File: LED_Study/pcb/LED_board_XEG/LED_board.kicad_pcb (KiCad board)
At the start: 2 copper layers, 25.4 x 25.4 mm, 4 parts

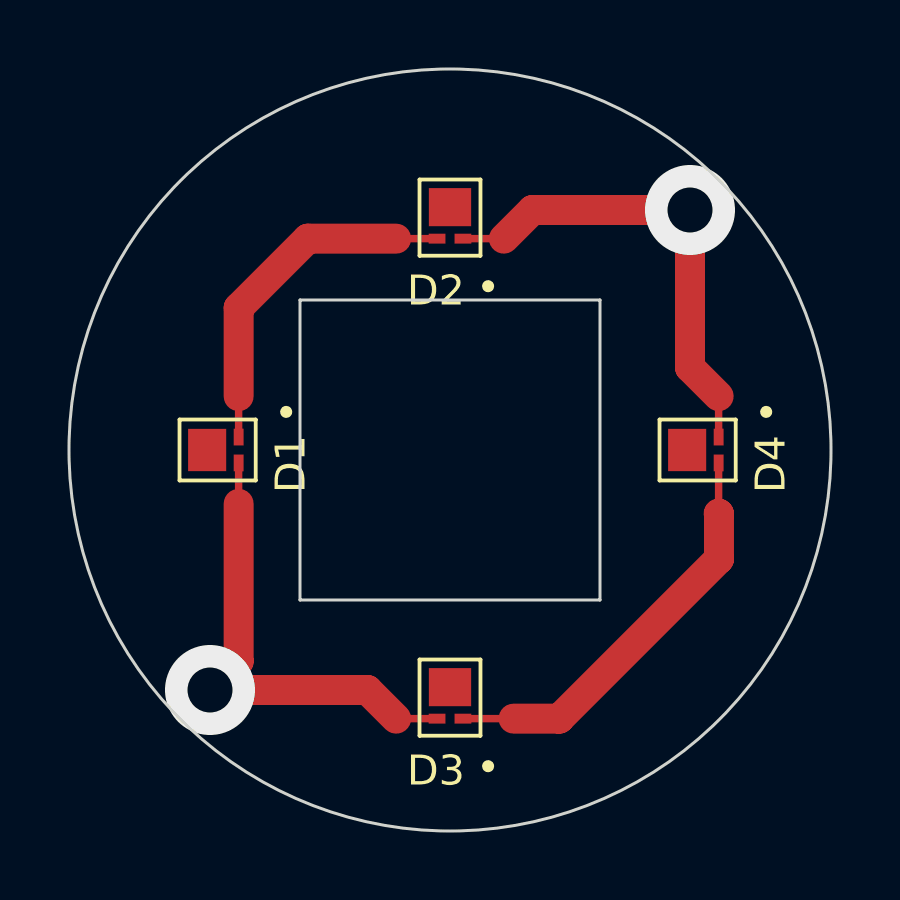
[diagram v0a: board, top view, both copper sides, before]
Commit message: new boards
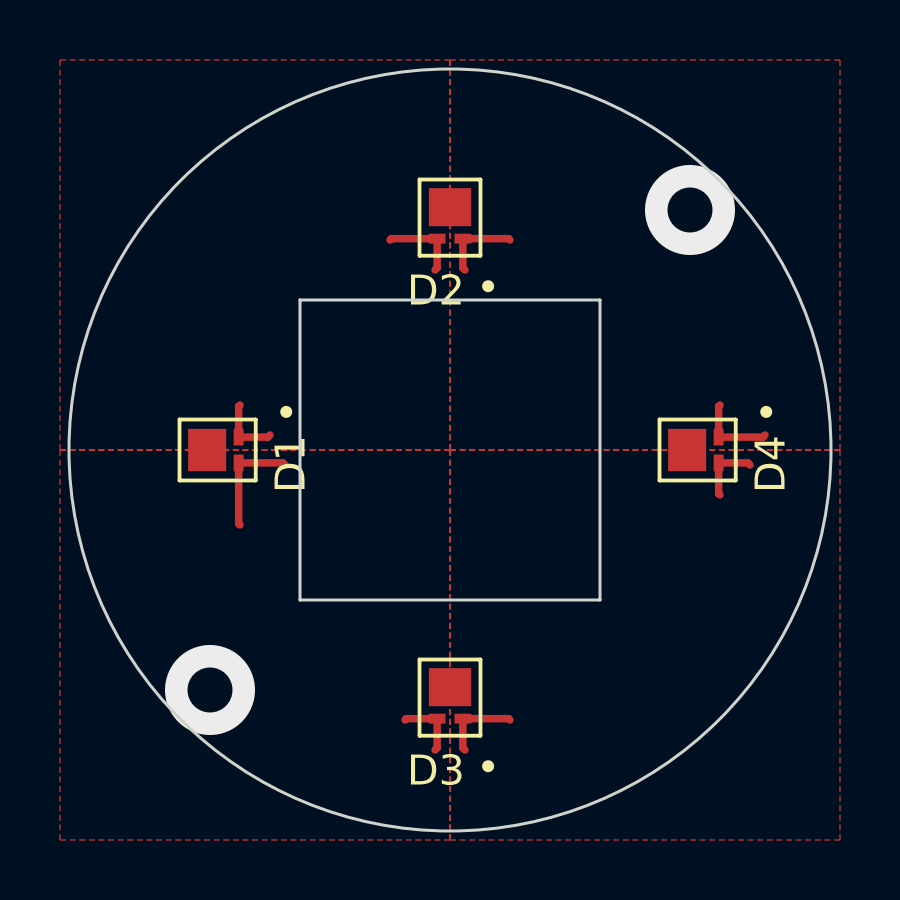
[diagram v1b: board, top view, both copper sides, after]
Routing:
- net /GND: track 15.9 -> 5.33 mm
- net /Vin: track 15.9 -> 5.83 mm
- net Net-(D3-Pad1): track 13.9 -> 4.83 mm
- net Net-(D1-Pad1): track 11.9 -> 4.83 mm
- added copper zone on F.Cu, net /GND
- added copper zone on F.Cu, net /Vin
- added copper zone on F.Cu, net Net-(D1-Pad1)
- added copper zone on F.Cu, net Net-(D3-Pad1)
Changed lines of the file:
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@@
   (gr_circle (center 100 100) (end 112.7 100)
     (stroke (width 0.1) (type default)) (fill none) (layer "Edge.Cuts"))
-  (segment (start 92.955 95.259) (end 95.259 92.955) (width 1) (layer "F.Cu") (net 1))
-  (segment (start 95.259 92.955) (end 98.205 92.955) (width 1) (layer "F.Cu") (net 1))
-  (segment (start 99.57 92.955) (end 98.205 92.955) (width 0.25) (layer "F.Cu") (net 1))
-  (segment (start 92.955 99.57) (end 92.955 98.205) (width 0.25) (layer "F.Cu") (net 1))
-  (segment (start 92.955 98.205) (end 92.955 95.259) (width 1) (layer "F.Cu") (net 1))
-  (segment (start 98.205 108.955) (end 97.25 108) (width 1) (layer "F.Cu") (net 3))
-  (segment (start 92.955 101.795) (end 92.955 107.045) (width 1) (layer "F.Cu") (net 3))
-  (segment (start 92.955 107.045) (end 92 108) (width 1) (layer "F.Cu") (net 3))
-  (segment (start 92.955 100.43) (end 92.955 101.795) (width 0.25) (layer "F.Cu") (net 3))
-  (segment (start 97.25 108) (end 92 108) (width 1) (layer "F.Cu") (net 3))
-  (segment (start 99.57 108.955) (end 98.205 108.955) (width 0.25) (layer "F.Cu") (net 3))
+  (segment (start 99.57 92.955) (end 99.57 93.93) (width 0.25) (layer "F.Cu") (net 1))
+  (segment (start 92.955 98.545) (end 93 98.5) (width 0.25) (layer "F.Cu") (net 1))
+  (segment (start 92.955 99.57) (end 92.955 98.545) (width 0.25) (layer "F.Cu") (net 1))
+  (segment (start 99.57 93.93) (end 99.5 94) (width 0.25) (layer "F.Cu") (net 1))
+  (segment (start 98.045 92.955) (end 98 93) (width 0.25) (layer "F.Cu") (net 1))
+  (segment (start 93.93 99.57) (end 94 99.5) (width 0.25) (layer "F.Cu") (net 1))
+  (segment (start 92.955 99.57) (end 93.93 99.57) (width 0.25) (layer "F.Cu") (net 1))
+  (segment (start 99.57 92.955) (end 98.045 92.955) (width 0.25) (layer "F.Cu") (net 1))
+  (segment (start 99.57 108.955) (end 98.545 108.955) (width 0.25) (layer "F.Cu") (net 3))
+  (segment (start 94.43 100.43) (end 94.5 100.5) (width 0.25) (layer "F.Cu") (net 3))
+  (segment (start 98.545 108.955) (end 98.5 109) (width 0.25) (layer "F.Cu") (net 3))
+  (segment (start 92.955 100.43) (end 94.43 100.43) (width 0.25) (layer "F.Cu") (net 3))
+  (segment (start 92.955 100.43) (end 92.955 102.455) (width 0.25) (layer "F.Cu") (net 3))
+  (segment (start 99.57 108.955) (end 99.57 109.93) (width 0.25) (layer "F.Cu") (net 3))
+  (segment (start 99.57 109.93) (end 99.5 110) (width 0.25) (layer "F.Cu") (net 3))
+  (segment (start 92.955 102.455) (end 93 102.5) (width 0.25) (layer "F.Cu") (net 3))
   (via (at 92 108) (size 3) (drill 1.5) (layers "F.Cu" "B.Cu") (free) (net 3))
-  (segment (start 108 92) (end 102.75 92) (width 1) (layer "F.Cu") (net 4))
-  (segment (start 108 92) (end 108 97.25) (width 1) (layer "F.Cu") (net 4))
-  (segment (start 108.955 98.205) (end 108 97.25) (width 1) (layer "F.Cu") (net 4))
-  (segment (start 101.795 92.955) (end 102.75 92) (width 1) (layer "F.Cu") (net 4))
-  (segment (start 108.955 99.57) (end 108.955 98.205) (width 0.25) (layer "F.Cu") (net 4))
-  (segment (start 100.43 92.955) (end 101.795 92.955) (width 0.25) (layer "F.Cu") (net 4))
+  (segment (start 100.43 92.955) (end 100.43 93.93) (width 0.25) (layer "F.Cu") (net 4))
+  (segment (start 108.955 99.57) (end 110.43 99.57) (width 0.25) (layer "F.Cu") (net 4))
+  (segment (start 108.955 98.545) (end 109 98.5) (width 0.25) (layer "F.Cu") (net 4))
+  (segment (start 100.43 93.93) (end 100.5 94) (width 0.25) (layer "F.Cu") (net 4))
+  (segment (start 100.43 92.955) (end 101.955 92.955) (width 0.25) (layer "F.Cu") (net 4))
+  (segment (start 110.43 99.57) (end 110.5 99.5) (width 0.25) (layer "F.Cu") (net 4))
+  (segment (start 101.955 92.955) (end 102 93) (width 0.25) (layer "F.Cu") (net 4))
+  (segment (start 108.955 99.57) (end 108.955 98.545) (width 0.25) (layer "F.Cu") (net 4))
   (via (at 108 92) (size 3) (drill 1.5) (layers "F.Cu" "B.Cu") (free) (net 4))
-  (segment (start 108.966 103.632) (end 103.643 108.955) (width 1) (layer "F.Cu") (net 6))
-  (segment (start 108.966 102.13) (end 108.966 103.632) (width 1) (layer "F.Cu") (net 6))
-  (segment (start 100.43 108.955) (end 102.119 108.955) (width 0.25) (layer "F.Cu") (net 6))
-  (segment (start 108.955 102.119) (end 108.966 102.13) (width 1) (layer "F.Cu") (net 6))
-  (segment (start 108.955 100.43) (end 108.955 102.119) (width 0.25) (layer "F.Cu") (net 6))
-  (segment (start 103.643 108.955) (end 102.119 108.955) (width 1) (layer "F.Cu") (net 6))
+  (segment (start 100.43 108.955) (end 100.43 109.93) (width 0.25) (layer "F.Cu") (net 6))
+  (segment (start 108.955 101.455) (end 109 101.5) (width 0.25) (layer "F.Cu") (net 6))
+  (segment (start 101.955 108.955) (end 102 109) (width 0.25) (layer "F.Cu") (net 6))
+  (segment (start 109.93 100.43) (end 110 100.5) (width 0.25) (layer "F.Cu") (net 6))
+  (segment (start 100.43 108.955) (end 101.955 108.955) (width 0.25) (layer "F.Cu") (net 6))
+  (segment (start 108.955 100.43) (end 109.93 100.43) (width 0.25) (layer "F.Cu") (net 6))
+  (segment (start 108.955 100.43) (end 108.955 101.455) (width 0.25) (layer "F.Cu") (net 6))
+  (segment (start 100.43 109.93) (end 100.5 110) (width 0.25) (layer "F.Cu") (net 6))
+  (zone (net 1) (net_name "Net-(D1-Pad1)") (layer "F.Cu") (hatch edge 0.5)
+    (priority 3)
+    (connect_pads (clearance 0.5))
+    (min_thickness 0.25) (filled_areas_thickness no)
+    (fill yes (thermal_gap 0.5) (thermal_bridge_width 0.5))
+    (polygon
+      (pts
+        (xy 100 100)
+        (xy 100 87)
+        (xy 87 87)
+        (xy 87 100)
+      )
+    )
+  )
+  (zone (net 4) (net_name "/GND") (layer "F.Cu") (hatch edge 0.5)
+    (connect_pads (clearance 0.5))
+    (min_thickness 0.25) (filled_areas_thickness no)
+    (fill yes (thermal_gap 0.5) (thermal_bridge_width 0.5))
+    (polygon
+      (pts
+        (xy 100 100)
+        (xy 100 87)
+        (xy 113 87)
+        (xy 113 100)
+      )
+    )
+  )
+  (zone (net 3) (net_name "/Vin") (layer "F.Cu") (hatch edge 0.5)
+    (priority 2)
+    (connect_pads (clearance 0.5))
+    (min_thickness 0.25) (filled_areas_thickness no)
+    (fill yes (thermal_gap 0.5) (thermal_bridge_width 0.5))
+    (polygon
+      (pts
+        (xy 100 100)
+        (xy 100 113)
+        (xy 87 113)
+        (xy 87 100)
+      )
+    )
+  )
+  (zone (net 6) (net_name "Net-(D3-Pad1)") (layer "F.Cu") (hatch edge 0.5)
+    (priority 1)
+    (connect_pads (clearance 0.5))
+    (min_thickness 0.25) (filled_areas_thickness no)
+    (fill yes (thermal_gap 0.5) (thermal_bridge_width 0.5))
+    (polygon
+      (pts
+        (xy 100 100)
+        (xy 113 100)
+        (xy 113 113)
+        (xy 100 113)
+      )
+    )
+  )
 )
